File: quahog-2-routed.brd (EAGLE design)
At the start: 68.5 x 17.9 mm, 33 parts, among them IC3 MCP1703CB, IC5 24AA128SN, J1 AYZ0202, X1 16 MHz

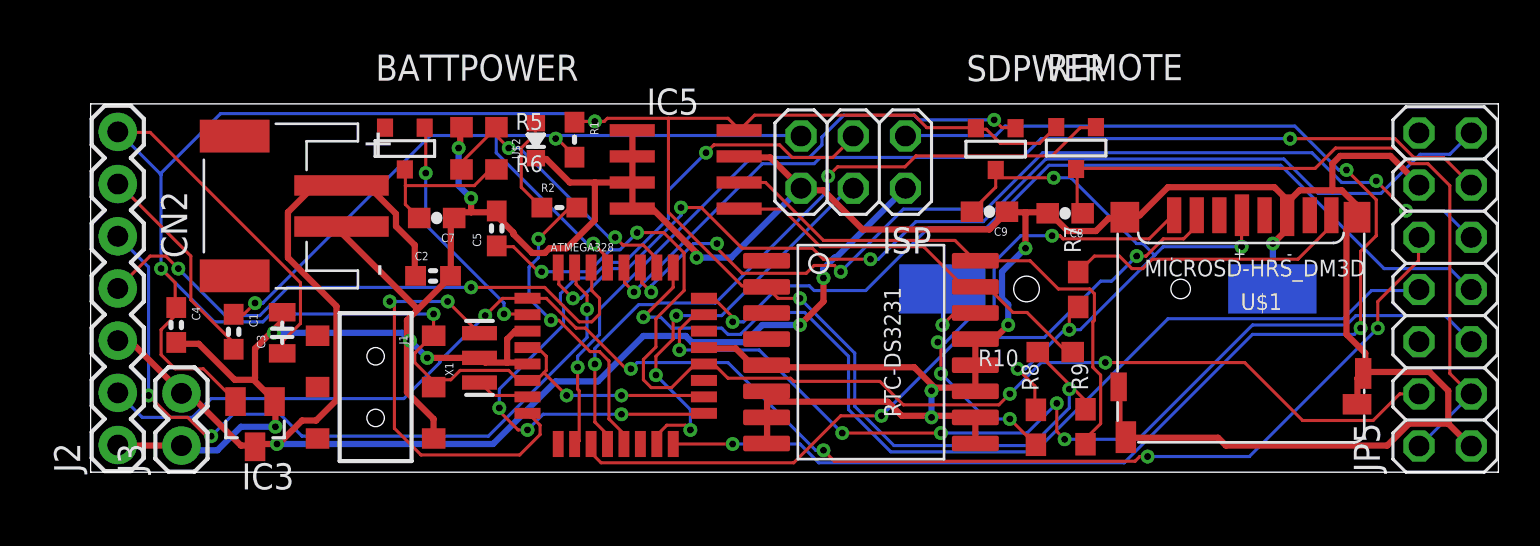
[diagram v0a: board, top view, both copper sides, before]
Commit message: update
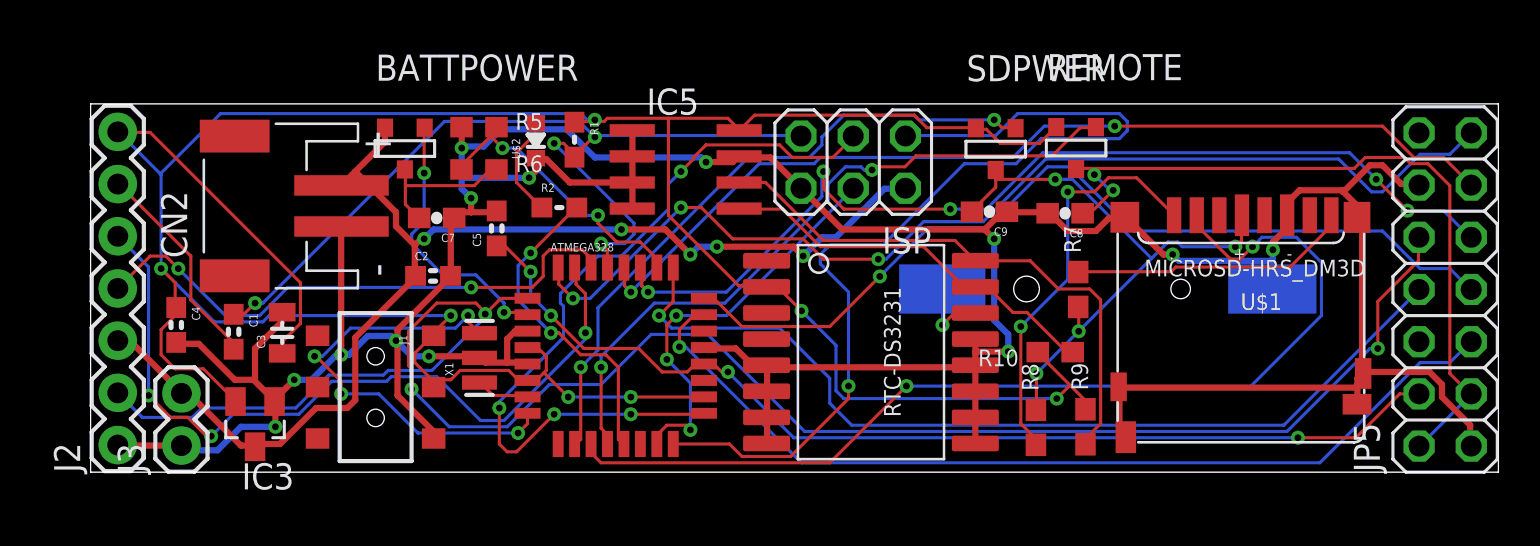
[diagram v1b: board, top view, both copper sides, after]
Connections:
- removed net VIN: BATTPOWER.2
- net PWR: now also BATTPOWER.2
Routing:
- net D12_MISO: track 67.7 -> 46.8 mm, vias 3 -> 1
- net GND: track 210.5 -> 195.0 mm, vias 12 -> 13
- net D7: track 35.4 -> 50.0 mm
- net D3: track 75.7 -> 89.9 mm, vias 5 -> 3
- net PWR: track 70.6 -> 58.4 mm, vias 3 -> 5
- net AREF: track 59.6 -> 50.6 mm
- net A2: track 49.2 -> 45.3 mm
- net N$18: track 23.3 -> 19.8 mm, vias 4 -> 2
- net RST: track 41.5 -> 43.8 mm, vias 3 -> 4
- net A0: track 47.8 -> 45.6 mm, vias 5 -> 1
- net D13_SCK: track 36.5 -> 38.3 mm
- net D0_RX: track 29.1 -> 27.4 mm
- net N$21: track 20.6 -> 22.3 mm, vias 2 -> 4
- net N$4: track 30.4 -> 28.7 mm
- net VCC: track 151.5 -> 150.0 mm
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
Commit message: update
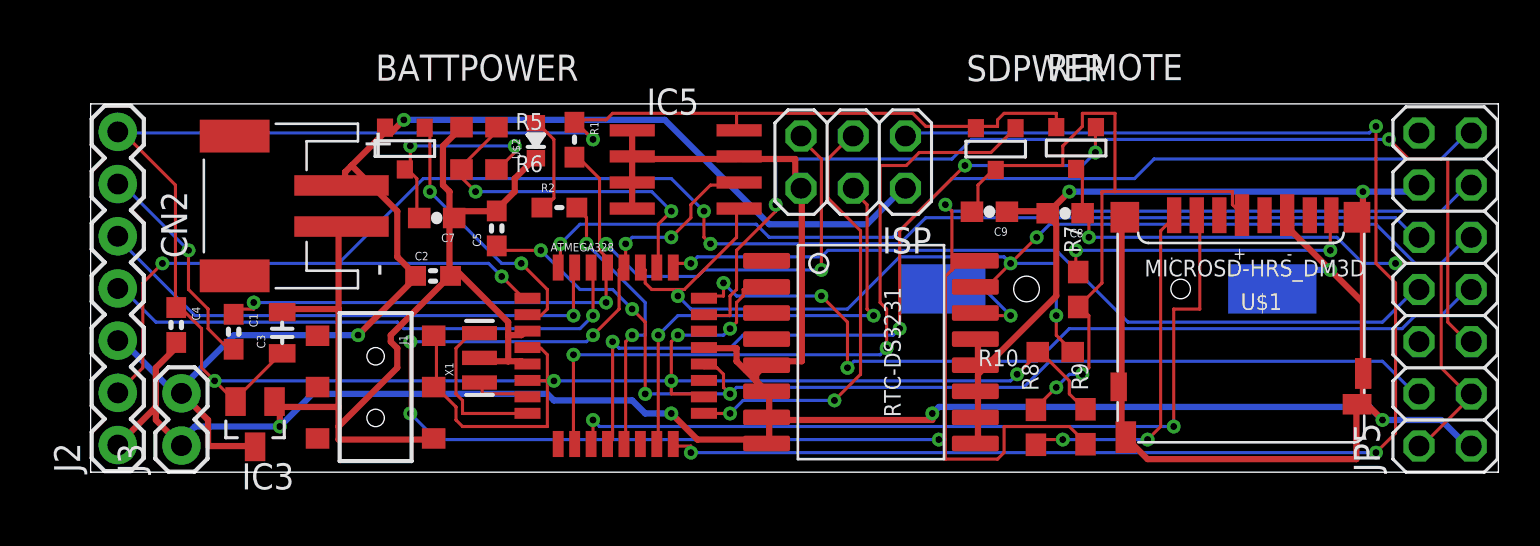
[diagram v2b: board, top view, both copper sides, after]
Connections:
- removed net A4_SDA: ATMEGA328.27, JP5.9
- removed net A5_SCL: ATMEGA328.28, JP5.11
- net SCL: now also ATMEGA328.28, JP5.11
- net SDA: now also ATMEGA328.27, JP5.9
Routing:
- net SCL: track 27.3 -> 100.2 mm, vias 0 -> 7
- net GND: track 195.0 -> 244.0 mm, vias 13 -> 7
- net A4_SDA: track 48.6 -> 0.00 mm, vias 5 -> 0
- net A5_SCL: track 46.8 -> 0.00 mm, vias 2 -> 0
- net SDA: track 19.2 -> 59.5 mm, vias 0 -> 4
- net D12_MISO: track 46.8 -> 74.3 mm, vias 1 -> 3
- net D13_SCK: track 38.3 -> 21.2 mm, vias 4 -> 2
- net N$21: track 22.3 -> 8.11 mm, vias 4 -> 0
- net D1_TX: track 37.9 -> 26.2 mm, vias 3 -> 1
- net VCC: track 150.0 -> 139.9 mm
- net D7: track 50.0 -> 41.2 mm
- net A0: track 45.6 -> 52.8 mm, vias 1 -> 2
- net D3: track 89.9 -> 82.9 mm, vias 3 -> 4
- net A2: track 45.3 -> 38.7 mm
- net N$4: track 28.7 -> 34.9 mm, vias 4 -> 2
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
